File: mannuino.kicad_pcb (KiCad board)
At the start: 2 copper layers, 27 x 33.8 mm, 24 parts, among them J1 USB_C_Receptacle_USB2.0_16P, J2 Conn_01x13, J3 Conn_01x15, J4 Conn_01x15, SW1 SW_Push, SW2 SW_Push, U2 USBLC6-2SC6, U3 XC6220B331MR, U4 ESP32-S3-WROOM-2

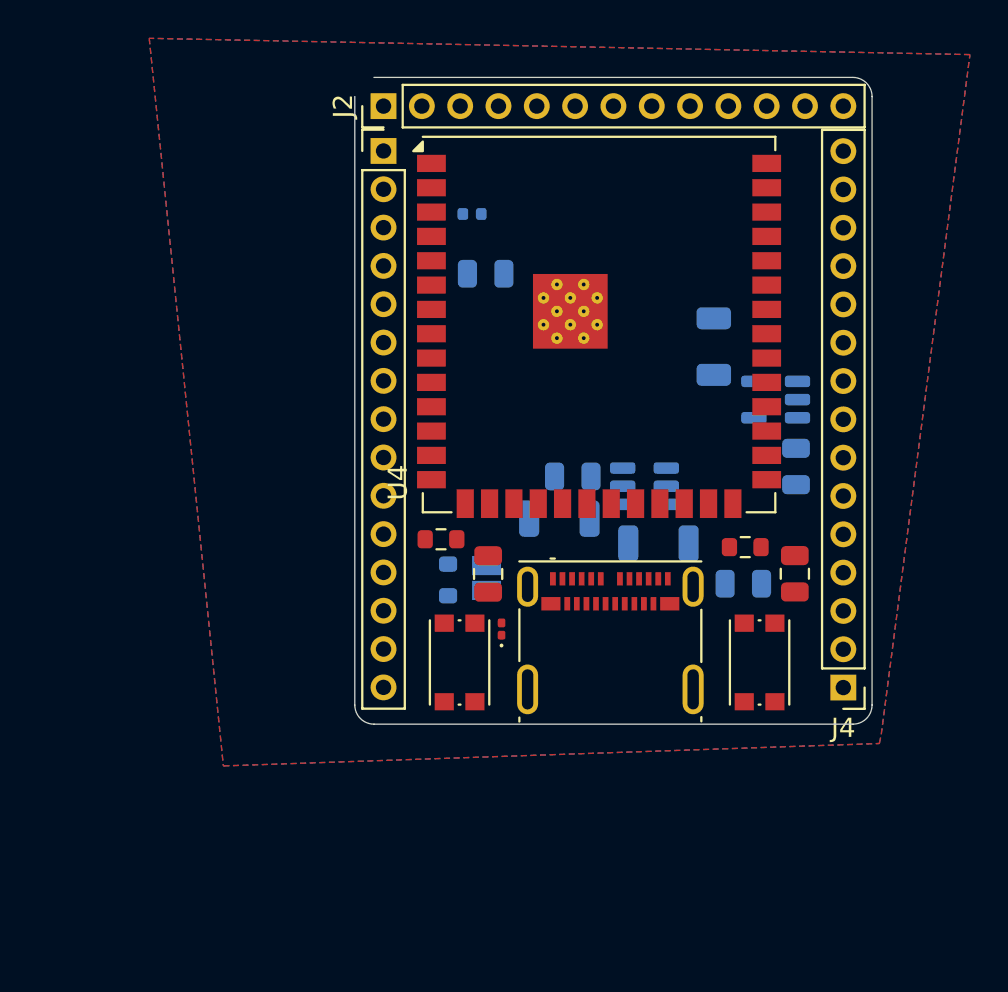
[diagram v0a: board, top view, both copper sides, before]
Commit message: IG last version
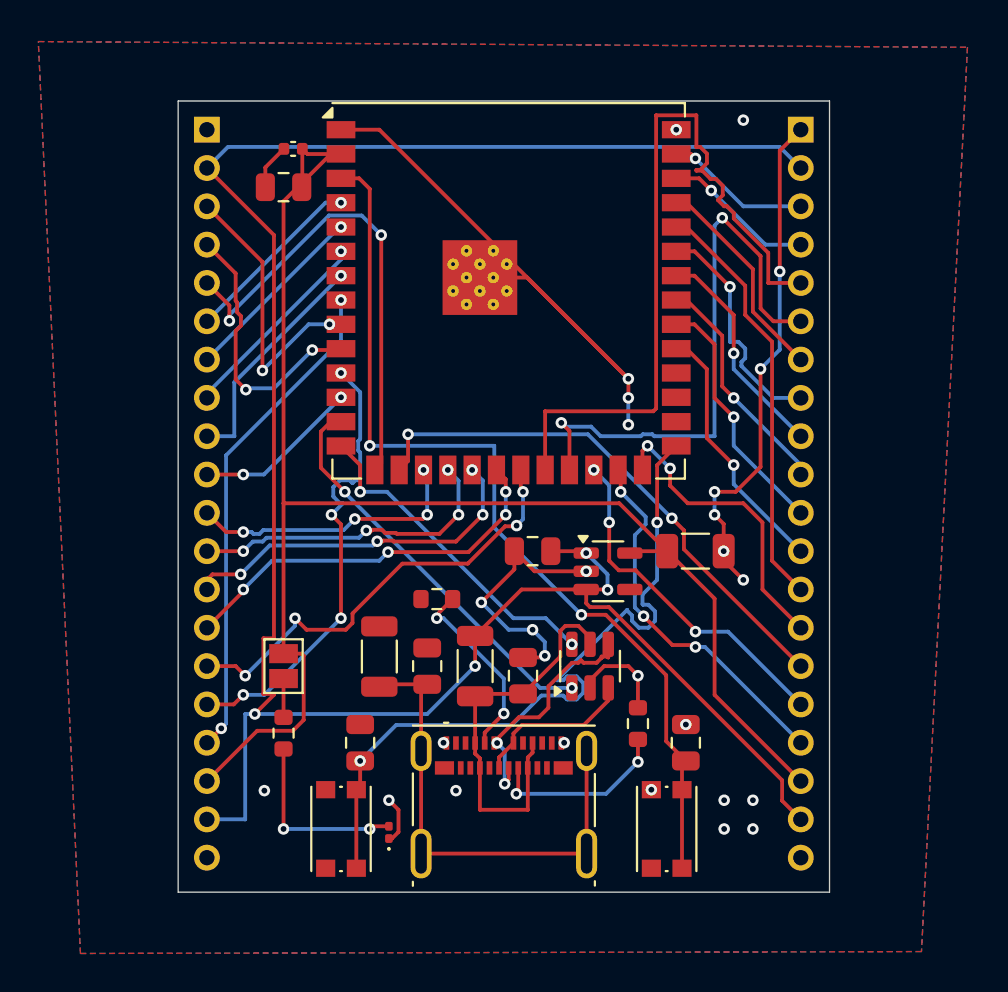
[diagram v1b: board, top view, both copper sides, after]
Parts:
- removed J4: Conn_01x15, Connector_PinHeader_2.00mm:PinHeader_1x15_P2.00mm_Vertical
- C4, C5, C6, C7, C8, C9, FB1, FB2, JP1, R4, U2, U3: moved to F.Cu
- J2: value Conn_01x13 -> Conn_01x20; footprint Connector_PinHeader_2.00mm:PinHeader_1x13_P2.00mm_Vertical -> Connector_PinHeader_2.00mm:PinHeader_1x20_P2.00mm_Vertical; moved to B.Cu
- J3: value Conn_01x15 -> Conn_01x20; footprint Connector_PinHeader_2.00mm:PinHeader_1x15_P2.00mm_Vertical -> Connector_PinHeader_2.00mm:PinHeader_1x20_P2.00mm_Vertical; moved to B.Cu
- moved J2 21.8 mm to (96.0, 23.0), turned to 180 degrees
- moved C5 17.1 mm to (76.5, 51.0), turned to 90 degrees
- moved FB2 15.7 mm to (74.0, 50.5), turned to -90 degrees
- moved C6 14.4 mm to (82.0, 45.0), turned to 180 degrees
- moved U3 12.5 mm to (85.9, 46.0), turned to 0 degrees
- moved D2 12.1 mm to (74.5, 59.7)
- moved R4 11.7 mm to (69.0, 54.5)
- moved JP1 11.6 mm to (69.0, 51.0), turned to 90 degrees
- moved C9 11.5 mm to (69.0, 26.0), turned to 180 degrees
- moved C3 11.1 mm to (73.0, 55.0)
- moved R2 10.8 mm to (87.5, 54.0), turned to 90 degrees
- moved C7 10.7 mm to (90.5, 45.0), turned to 0 degrees
- moved C4 10.7 mm to (81.5, 51.5), turned to 90 degrees
- moved SW2 10.7 mm to (72.0, 59.5)
- moved C2 10.5 mm to (90.0, 55.0)
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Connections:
- J2 pad 1: +5V -> GND
- J2 pad 10: GND -> /GPIO22
- J2 pad 11: GND -> /GPIO21
- J2 pad 12: GND -> /GPIO20
- J2 pad 13: GND -> /GPIO26
- J2 pad 3: +5V -> /GPIO0
- J2 pad 4: +5V -> /GPIO1
- J2 pad 5: +5V -> /GPIO14
- J2 pad 6: +3V3 -> /GPIO19
- J2 pad 7: +3V3 -> /GPIO25
- J2 pad 8: +3V3 -> /GPIO24
- J2 pad 9: +3V3 -> /GPIO23
- J3 pad 1: /GPIO0 -> GND
- J3 pad 10: /GPIO9 -> /GPIO7
- J3 pad 11: /GPIO11 -> /GPIO8
- J3 pad 12: /GPIO12 -> /GPIO9
- J3 pad 13: /GPIO13 -> /GPIO11
- J3 pad 14: /GPIO14 -> /GPIO12
- J3 pad 15: /GPIO15 -> /GPIO13
- J3 pad 2: /GPIO1 -> +5V
- J3 pad 3: /GPIO2 -> /GPIO16
- J3 pad 4: /GPIO3 -> /GPIO17
- J3 pad 5: /GPIO4 -> /GPIO2
- J3 pad 6: /GPIO5 -> /GPIO3
- J3 pad 7: /GPIO6 -> /GPIO4
- J3 pad 8: /GPIO7 -> /GPIO5
- J3 pad 9: /GPIO8 -> /GPIO6
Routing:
- net +5V: track 0.00 -> 115.9 mm, vias 0 -> 4
- net GND: track 0.00 -> 83.3 mm, vias 0 -> 27
- net +3V3: track 0.00 -> 80.5 mm
- net /en: track 0.00 -> 48.7 mm, vias 0 -> 2
- net /GPIO14: track 0.00 -> 39.7 mm
- net /boot: track 0.00 -> 38.8 mm, vias 0 -> 2
- net /GPIO19: track 0.00 -> 30.5 mm, vias 0 -> 2
- net /GPIO28: track 0.00 -> 28.1 mm, vias 0 -> 2
- net /GPIO15: track 0.00 -> 26.0 mm, vias 0 -> 2
- net /GPIO2: track 0.00 -> 25.7 mm, vias 0 -> 2
- net Net-(J1-SHIELD): track 0.00 -> 25.5 mm
- net /GPIO18: track 0.00 -> 24.2 mm, vias 0 -> 4
- net /GPIO13: track 0.00 -> 23.7 mm, vias 0 -> 4
- net /GPIO26: track 0.00 -> 21.9 mm
- net /USB_D-: track 0.00 -> 21.0 mm, vias 0 -> 2
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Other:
- board size 27 x 33.8 mm -> 34 x 41.3 mm
